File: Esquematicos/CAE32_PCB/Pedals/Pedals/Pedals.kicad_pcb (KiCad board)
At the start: 4 copper layers, 76.1 x 70.2 mm, 132 parts, among them J1 SPI_MASTER, J10 Conn_01x03_Female, J11 Conn_01x03_Female, J12 Conn_01x03_Female, J13 Conn_01x03_Female, J14 Conn_01x03_Female, J15 USB_C_Receptacle_USB2.0, J16 UART_PGR, J18 LC, J19 LC, J2 CAN, J20 LC, J3 PGRM and SPI, J4 Conn_01x03_Female, J5 Conn_01x03_Female, J6 Conn_01x03_Female, J7 Conn_01x03_Female, J8 Conn_01x03_Female, J9 Conn_01x03_Female, Q1 MMBT3906, Q2 MMBT3906, Q3 MMBT3906, SW1 CONFIG, SW2 SW, SW3 SW, U1 STM32F072RBTx, U2 REF3033, U3 ADC128S022, U4 LDL1117, U5 HX711, U6 HX711, U7 HX711

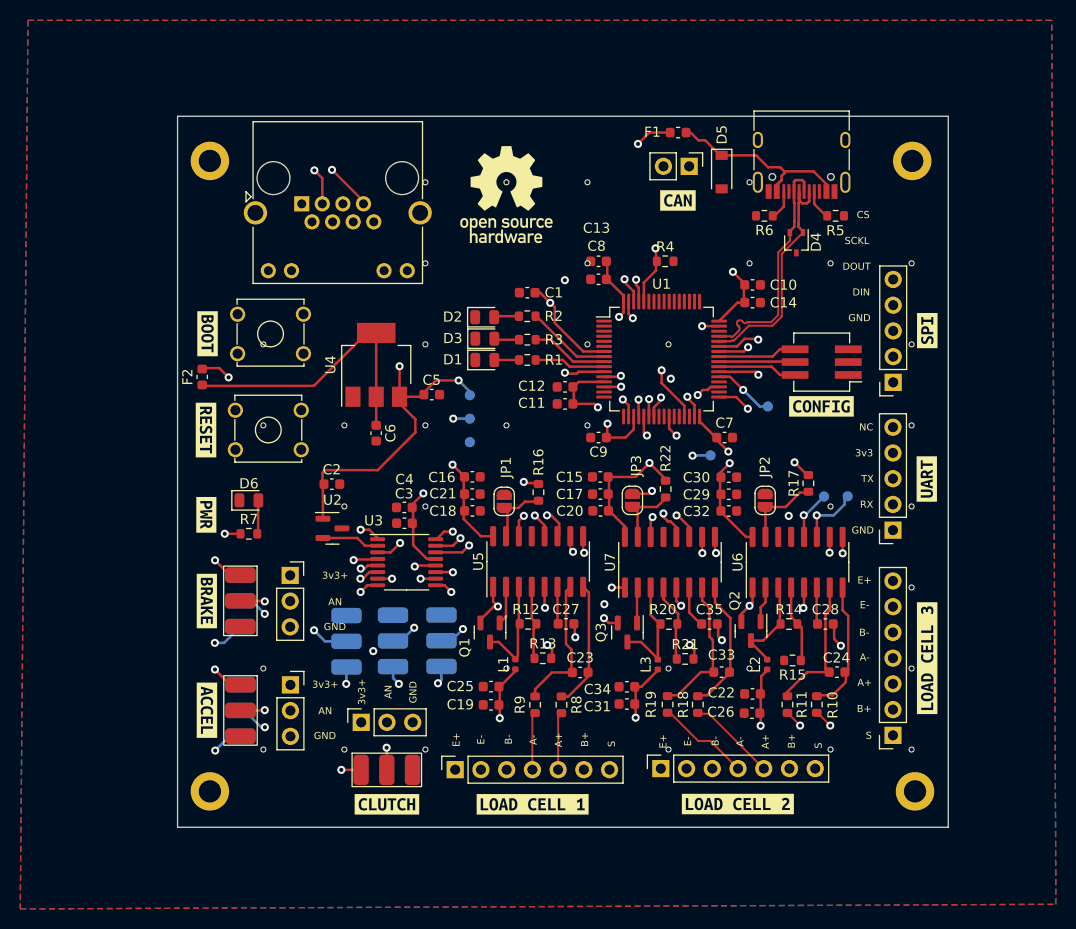
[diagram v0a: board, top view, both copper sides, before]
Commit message: update: PCB pedals Version:2.1.1
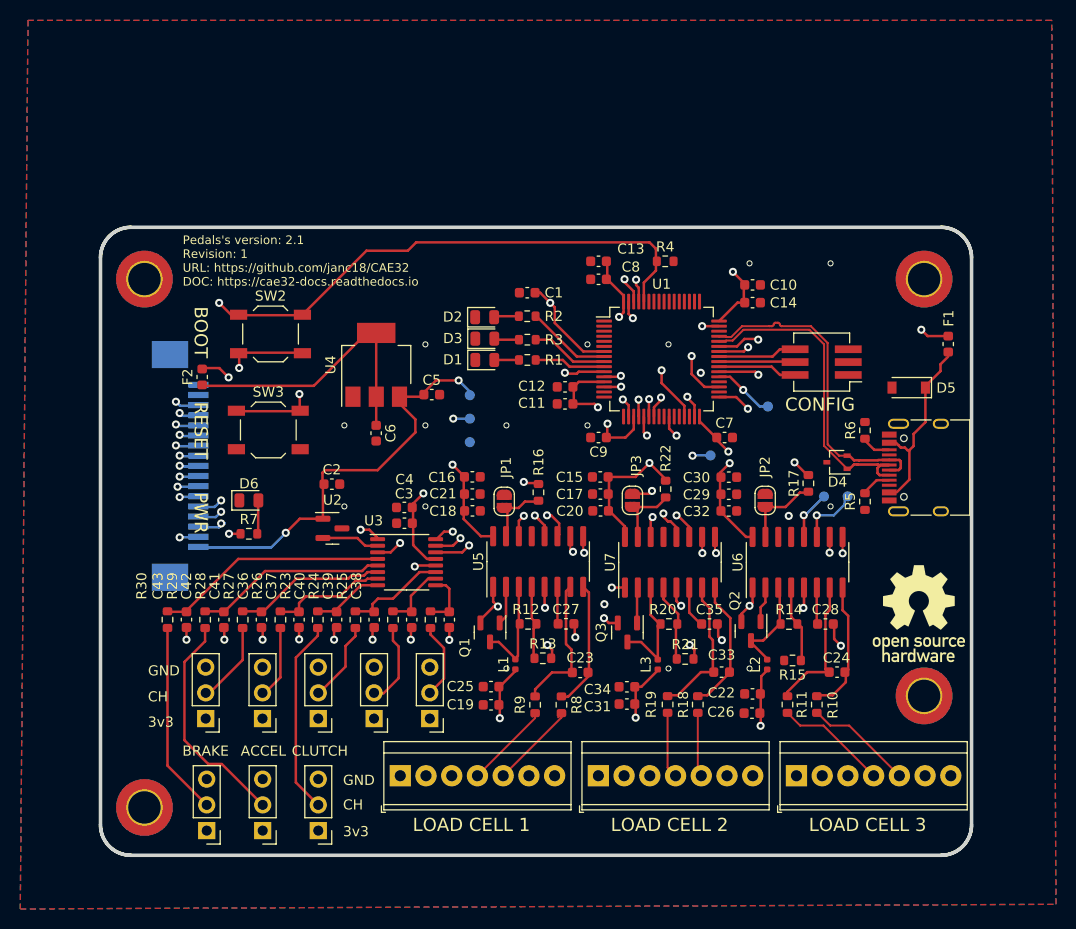
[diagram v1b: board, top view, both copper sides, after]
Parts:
- removed J12, J4, J8: Conn_01x03_Female, Connector_PinSocket_2.54mm:PinSocket_1x03_P2.54mm_Vertical
- removed J16: UART_PGR, Connector_PinSocket_2.54mm:PinSocket_1x05_P2.54mm_Vertical
- removed J2: CAN, Connector_PinHeader_2.54mm:PinHeader_1x02_P2.54mm_Vertical
- removed J20: LC, Connector_PinSocket_2.54mm:PinSocket_1x07_P2.54mm_Vertical
- removed J3: PGRM and SPI, Connector_RJ:RJ45_Amphenol_RJHSE538X
- removed kibuzzard-649339C9: G***, kibuzzard-649339C9
- removed kibuzzard-64933A47: G***, kibuzzard-64933A47
- removed kibuzzard-64933AAF: G***, kibuzzard-64933AAF
- removed kibuzzard-64933E22: G***, kibuzzard-64933E22
- removed kibuzzard-64934685: G***, kibuzzard-64934685
- removed kibuzzard-64934750: G***, kibuzzard-64934750
- removed kibuzzard-64934CFB: G***, kibuzzard-64934CFB
- removed kibuzzard-64934D05: G***, kibuzzard-64934D05
- removed kibuzzard-64935B19: G***, kibuzzard-64935B19
- removed kibuzzard-64935FC0: G***, kibuzzard-64935FC0
- removed kibuzzard-649360F1: G***, kibuzzard-649360F1
- removed kibuzzard-649361A8: G***, kibuzzard-649361A8
- removed kibuzzard-64936236: G***, kibuzzard-64936236
- removed kibuzzard-64936313: G***, kibuzzard-64936313
- removed kibuzzard-64936394: G***, kibuzzard-64936394
- removed kibuzzard-6493639C: G***, kibuzzard-6493639C
- removed kibuzzard-649363C1: G***, kibuzzard-649363C1
- removed kibuzzard-649363D8: G***, kibuzzard-649363D8
- added C36: 33n, Capacitor_SMD:C_0603_1608Metric, F.Cu at (117.5, 112.1)
- added C37: 33n, Capacitor_SMD:C_0603_1608Metric, F.Cu at (121.2, 112.1)
- added C38: 33n, Capacitor_SMD:C_0603_1608Metric, F.Cu at (132.3, 112.1)
- added C39: 33n, Capacitor_SMD:C_0603_1608Metric, F.Cu at (128.6, 112.1)
- added C40: 33n, Capacitor_SMD:C_0603_1608Metric, F.Cu at (124.9, 112.1)
- added C41: 33n, Capacitor_SMD:C_0603_1608Metric, F.Cu at (113.8, 112.1)
- added C42: 33n, Capacitor_SMD:C_0603_1608Metric, F.Cu at (110.1, 112.1)
- added C43: 33n, Capacitor_SMD:C_0603_1608Metric, F.Cu at (106.4, 112.1)
- added J17: LC, TerminalBlock_TE-Connectivity:TerminalBlock_TE_282834-7_1x07_P2.54mm_Horizontal, F.Cu at (166.6, 127.5)
- added R23: 100, Resistor_SMD:R_0603_1608Metric, F.Cu at (123.1, 112.1)
- added R24: 100, Resistor_SMD:R_0603_1608Metric, F.Cu at (126.8, 112.1)
- added R25: 100, Resistor_SMD:R_0603_1608Metric, F.Cu at (130.5, 112.1)
- added R26: 100, Resistor_SMD:R_0603_1608Metric, F.Cu at (119.4, 112.1)
- added R27: 100, Resistor_SMD:R_0603_1608Metric, F.Cu at (115.7, 112.1)
- added R28: 100, Resistor_SMD:R_0603_1608Metric, F.Cu at (111.9, 112.1)
- added R29: 100, Resistor_SMD:R_0603_1608Metric, F.Cu at (108.2, 112.1)
- added R30: 100, Resistor_SMD:R_0603_1608Metric, F.Cu at (104.5, 112.1)
- H1, H2, H3, H4: footprint MountingHole:MountingHole_2.2mm_M2_DIN965_Pad -> MountingHole:MountingHole_3.2mm_M3_DIN965_Pad_TopBottom
- J1: value SPI_MASTER -> Conn_01x19_Pin; footprint Connector_PinSocket_2.54mm:PinSocket_1x05_P2.54mm_Vertical -> Connector_FFC-FPC:TE_1-84953-7_1x17-1MP_P1.0mm_Horizontal; moved to B.Cu
- J10, J11, J14, J6, J7: footprint Extra_components:1x3_pin -> Connector_PinHeader_2.54mm:PinHeader_1x03_P2.54mm_Vertical; moved to F.Cu
- J13, J5, J9: footprint Extra_components:1x3_pin -> Connector_PinHeader_2.54mm:PinHeader_1x03_P2.54mm_Vertical
- J18, J19: footprint Connector_PinSocket_2.54mm:PinSocket_1x07_P2.54mm_Vertical -> TerminalBlock_TE-Connectivity:TerminalBlock_TE_282834-7_1x07_P2.54mm_Horizontal
- SW2, SW3: footprint Extra_components:TS-1095PD-A16B2-D2 -> Button_Switch_SMD:SW_SPST_TL3342
- moved J1 70.9 mm to (105.8, 96.9), turned to 90 degrees
- moved J19 48.8 mm to (127.5, 127.5), turned to 0 degrees
- moved F1 33.9 mm to (181.6, 84.9), turned to 90 degrees
- moved J15 33.8 mm to (179.8, 97.1), turned to 90 degrees
- moved R5 28.4 mm to (173.4, 100.4), turned to -90 degrees
- moved D5 28.2 mm to (177.7, 89.2), turned to 180 degrees
- moved R6 23.4 mm to (173.4, 93.4), turned to 90 degrees
- moved J5 22.9 mm to (108.4, 132.9), turned to 180 degrees
- moved D4 22.0 mm to (170.6, 96.6), turned to 180 degrees
- moved J6 14.4 mm to (119.4, 121.9), turned to 180 degrees
- moved J18 14.1 mm to (147.1, 127.5), turned to 0 degrees
- moved H3 13.3 mm to (102.2, 78.5)
- moved J9 12.1 mm to (113.9, 132.9), turned to 180 degrees
- moved J11 11.8 mm to (113.9, 121.9), turned to 180 degrees
- moved H4 11.7 mm to (179.2, 78.5)
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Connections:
- C19 pad 1: Net-(J18-Pin_7) -> Net-(J19-Pin_7)
- C22 pad 1: Net-(J19-Pin_7) -> Net-(J17-Pin_7)
- C25 pad 1: Net-(J18-Pin_7) -> Net-(J19-Pin_7)
- C26 pad 1: Net-(J19-Pin_7) -> Net-(J17-Pin_7)
- C31 pad 1: Net-(J20-Pin_7) -> Net-(J18-Pin_7)
- C34 pad 1: Net-(J20-Pin_7) -> Net-(J18-Pin_7)
- J1 pad 1: GNDREF -> +5V
- J1 pad 2: /DIN -> +3.3V
- J1 pad 3: /DOUT -> /S_CKL
- J1 pad 4: /SCKL -> /S_CS_PEDALS
- J1 pad 5: /CS_ADC -> /S_DIN
- J10 pad 2: /ADCs components/Custom_2 -> /ADCs components/CH_2
- J11 pad 2: /ADCs components/Custom_5 -> /ADCs components/CH_5
- J14 pad 2: /ADCs components/Custom_3 -> /ADCs components/CH_3
- J18 pad 2: /Load Cells/B2+ -> /Load Cells/B3+
- J18 pad 3: /Load Cells/B2- -> /Load Cells/B3-
- J18 pad 4: /Load Cells/A2- -> /Load Cells/A3-
- J18 pad 5: /Load Cells/A2+ -> /Load Cells/A3+
- J19 pad 2: /Load Cells/B1+ -> /Load Cells/B2+
- J19 pad 3: /Load Cells/B1- -> /Load Cells/B2-
- J19 pad 4: /Load Cells/A1- -> /Load Cells/A2-
- J19 pad 5: /Load Cells/A1+ -> /Load Cells/A2+
- J6 pad 2: /ADCs components/Custom_1 -> /ADCs components/CH_1
- J7 pad 2: /ADCs components/Custom_4 -> /ADCs components/CH_4
- L1 pad 1: Net-(J18-Pin_7) -> Net-(J19-Pin_7)
- L2 pad 1: Net-(J19-Pin_7) -> Net-(J17-Pin_7)
- L3 pad 1: Net-(J20-Pin_7) -> Net-(J18-Pin_7)
- U3 pad 10: /ADCs components/Custom_2 -> /ADCs components/IN6
- U3 pad 11: /ADCs components/Custom_1 -> /ADCs components/IN7
- U3 pad 4: /ADCs components/BRAKE -> /ADCs components/IN0
- U3 pad 5: /ADCs components/ACCEL -> /ADCs components/IN1
- U3 pad 6: /ADCs components/CLUTCH -> /ADCs components/IN2
- U3 pad 7: /ADCs components/Custom_5 -> /ADCs components/IN3
- U3 pad 8: /ADCs components/Custom_4 -> /ADCs components/IN4
- U3 pad 9: /ADCs components/Custom_3 -> /ADCs components/IN5
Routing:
- net /PGR_UART_RX: track 25.3 -> 71.9 mm, vias 1 -> 2
- net /PGR_UART_TX: track 24.2 -> 69.3 mm, vias 1 -> 2
- net /CAN_TX: track 15.3 -> 55.4 mm, vias 1 -> 2
- net /CAN_RX: track 15.6 -> 55.4 mm, vias 1 -> 2
- net /ADCs components/Custom_4: track 28.9 -> 0.00 mm, vias 2 -> 0
- net Net-(J17-Pin_7): track 0.00 -> 26.6 mm, vias 0 -> 1
- net /ADCs components/Custom_3: track 26.3 -> 0.00 mm, vias 2 -> 0
- net Net-(J20-Pin_7): track 25.7 -> 0.00 mm, vias 1 -> 0
- net /ADCs components/IN0: track 0.00 -> 23.0 mm
- net /ADCs components/Custom_5: track 23.0 -> 0.00 mm, vias 2 -> 0
- net /DIN: track 63.6 -> 82.7 mm
- net /ADCs components/IN1: track 0.00 -> 18.9 mm
- net /S_DOUT: track 47.8 -> 63.5 mm, vias 1 -> 2
- net /ADCs components/IN2: track 0.00 -> 14.9 mm
- net /S_CS_PEDALS: track 52.7 -> 66.9 mm, vias 1 -> 3
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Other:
- board size 76.1 x 70.2 mm -> 86 x 62 mm
- board text added: "ACCEL"
- board text added: "BOOT"
- board text added: "BRAKE"
- board text added: "CH"
- board text added: "CLUTCH"
- board text added: "CONFIG"
- board text added: "LOAD CELL 1"
- board text added: "LOAD CELL 2"
- board text added: "LOAD CELL 3"
- board text added: "PWR"
- board text added: "Pedals's version: 2.1 Revision: 1 URL: https://github.com/janc18/CAE32 DOC: https://cae32-docs.readthedocs.io"
- board text added: "RESET"
- board text removed: "3v3+"
- board text removed: "A+"
- board text removed: "A-"
- board text removed: "AN"
- board text removed: "B+"
- board text removed: "B-"
- board text removed: "CS"
- board text removed: "DIN"
- board text removed: "DOUT"
- board text removed: "E+"
- board text removed: "E-"
- board text removed: "NC"
- board text removed: "Pedals's version: 2.0 Revision: 2 URL: https://github.com/janc18/CAE32"
- board text removed: "RX"
- board text removed: "S"
- board text removed: "SCKL"
- board text removed: "TX"
